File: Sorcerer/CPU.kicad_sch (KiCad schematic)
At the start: 35 parts

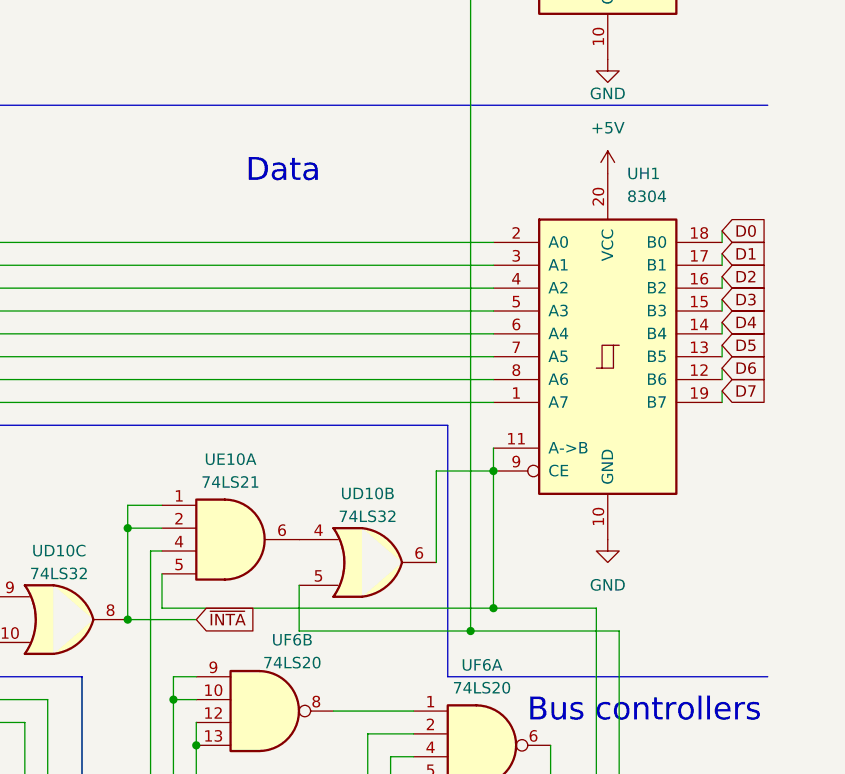
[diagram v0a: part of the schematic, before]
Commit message: Fix some issues I found.
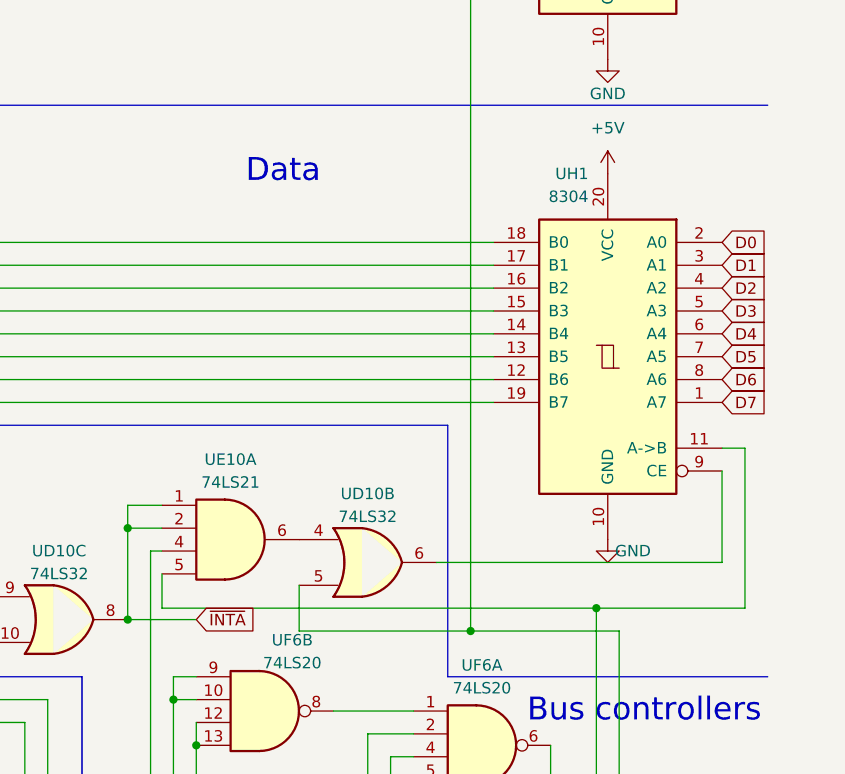
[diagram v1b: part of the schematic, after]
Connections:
- net D0: now also UH1.2 (A0); no longer UH1.18 (B0)
- net D1: now also UH1.3 (A1); no longer UH1.17 (B1)
- net D2: now also UH1.4 (A2); no longer UH1.16 (B2)
- net D3: now also UH1.5 (A3); no longer UH1.15 (B3)
- net D4: now also UH1.6 (A4); no longer UH1.14 (B4)
- net D5: now also UH1.7 (A5); no longer UH1.13 (B5)
- net D6: now also UH1.8 (A6); no longer UH1.12 (B6)
- net D7: now also UH1.1 (A7); no longer UH1.19 (B7)
- net ~{DBUS_OUT}: no longer UD10.6, UH1.9 (CE)
- net at UE2.10 (D_{6}): now also UH1.12 (B6); no longer UH1.8 (A6)
- net at UE2.12 (D_{2}): now also UH1.16 (B2); no longer UH1.4 (A2)
- net at UE2.13 (D_{7}): now also UH1.19 (B7); no longer UH1.1 (A7)
- net at UE2.14 (D_{0}): now also UH1.18 (B0); no longer UH1.2 (A0)
- net at UE2.15 (D_{1}): now also UH1.17 (B1); no longer UH1.3 (A1)
- net at UE2.7 (D_{4}): now also UH1.14 (B4); no longer UH1.6 (A4)
- net at UE2.8 (D_{3}): now also UH1.15 (B3); no longer UH1.5 (A3)
- net at UE2.9 (D_{5}): now also UH1.13 (B5); no longer UH1.7 (A5)
- new net: UD10.6, UH1.9 (CE)
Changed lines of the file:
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@@
 	)
 	(junction
-		(at 375.92 157.48)
-		(diameter 0)
-		(color 0 0 0 0)
-	)
-	(junction
 		(at 298.45 232.41)
 		(diameter 0)
@@
 	)
 	(junction
+		(at 387.35 172.72)
+		(diameter 0)
+		(color 0 0 0 0)
+	)
+	(junction
 		(at 260.35 257.81)
 		(diameter 0)
@@
 	)
 	(junction
-		(at 375.92 172.72)
-		(diameter 0)
-		(color 0 0 0 0)
-	)
-	(junction
 		(at 234.95 175.26)
 		(diameter 0)
@@
 	(wire
 		(pts
+			(xy 401.32 154.94) (xy 403.86 154.94)
+		)
+		(stroke
+			(width 0)
+			(type default)
+		)
+	)
+	(wire
+		(pts
 			(xy 264.16 255.27) (xy 267.97 255.27)
 		)
@@
 	(wire
 		(pts
-			(xy 387.35 172.72) (xy 375.92 172.72)
+			(xy 339.09 172.72) (xy 387.35 172.72)
 		)
 		(stroke
@@
 	(wire
 		(pts
-			(xy 401.32 139.7) (xy 401.32 138.43)
-		)
-		(stroke
-			(width 0)
-			(type default)
-		)
-	)
-	(wire
-		(pts
 			(xy 275.59 144.78) (xy 262.89 144.78)
 		)
@@
 	(wire
 		(pts
-			(xy 369.57 157.48) (xy 375.92 157.48)
-		)
-		(stroke
-			(width 0)
-			(type default)
-		)
-	)
-	(wire
-		(pts
 			(xy 156.21 252.73) (xy 156.21 245.11)
 		)
@@
 	(wire
 		(pts
+			(xy 369.57 167.64) (xy 401.32 167.64)
+		)
+		(stroke
+			(width 0)
+			(type default)
+		)
+	)
+	(wire
+		(pts
 			(xy 367.03 191.77) (xy 367.03 207.01)
 		)
@@
 	(wire
 		(pts
-			(xy 401.32 142.24) (xy 401.32 140.97)
-		)
-		(stroke
-			(width 0)
-			(type default)
-		)
-	)
-	(wire
-		(pts
 			(xy 267.97 152.4) (xy 262.89 152.4)
 		)
@@
 	(wire
 		(pts
-			(xy 401.32 149.86) (xy 401.32 148.59)
-		)
-		(stroke
-			(width 0)
-			(type default)
-		)
-	)
-	(wire
-		(pts
 			(xy 222.25 137.16) (xy 237.49 137.16)
 		)
@@
 	(wire
 		(pts
-			(xy 375.92 172.72) (xy 375.92 157.48)
-		)
-		(stroke
-			(width 0)
-			(type default)
-		)
-	)
-	(wire
-		(pts
 			(xy 265.43 27.94) (xy 265.43 154.94)
 		)
@@
 	(wire
 		(pts
-			(xy 401.32 137.16) (xy 401.32 135.89)
-		)
-		(stroke
-			(width 0)
-			(type default)
-		)
-	)
-	(wire
-		(pts
 			(xy 99.06 26.67) (xy 99.06 24.13)
 		)
@@
 	(wire
 		(pts
-			(xy 401.32 134.62) (xy 401.32 133.35)
-		)
-		(stroke
-			(width 0)
-			(type default)
-		)
-	)
-	(wire
-		(pts
 			(xy 219.71 142.24) (xy 237.49 142.24)
 		)
@@
 	(wire
 		(pts
-			(xy 401.32 132.08) (xy 401.32 130.81)
-		)
-		(stroke
-			(width 0)
-			(type default)
-		)
-	)
-	(wire
-		(pts
 			(xy 336.55 222.25) (xy 336.55 250.19)
 		)
@@
 	(wire
 		(pts
-			(xy 369.57 167.64) (xy 369.57 157.48)
-		)
-		(stroke
-			(width 0)
-			(type default)
-		)
-	)
-	(wire
-		(pts
 			(xy 280.67 35.56) (xy 280.67 139.7)
 		)
@@
 	(wire
 		(pts
+			(xy 403.86 154.94) (xy 403.86 172.72)
+		)
+		(stroke
+			(width 0)
+			(type default)
+		)
+	)
+	(wire
+		(pts
 			(xy 25.4 45.72) (xy 35.56 45.72)
 		)
@@
 	(wire
 		(pts
-			(xy 401.32 147.32) (xy 401.32 146.05)
-		)
-		(stroke
-			(width 0)
-			(type default)
-		)
-	)
-	(wire
-		(pts
 			(xy 303.53 232.41) (xy 303.53 241.3)
 		)
@@
 	(wire
 		(pts
+			(xy 401.32 167.64) (xy 401.32 157.48)
+		)
+		(stroke
+			(width 0)
+			(type default)
+		)
+	)
+	(wire
+		(pts
 			(xy 323.85 207.01) (xy 367.03 207.01)
 		)
@@
 	(wire
 		(pts
-			(xy 401.32 144.78) (xy 401.32 143.51)
+			(xy 403.86 172.72) (xy 387.35 172.72)
 		)
 		(stroke
@@
 	(wire
 		(pts
-			(xy 375.92 157.48) (xy 375.92 154.94)
-		)
-		(stroke
-			(width 0)
-			(type default)
-		)
-	)
-	(wire
-		(pts
 			(xy 127 57.15) (xy 127 58.42)
 		)
@@
 	(wire
 		(pts
-			(xy 339.09 172.72) (xy 375.92 172.72)
-		)
-		(stroke
-			(width 0)
-			(type default)
-		)
-	)
-	(wire
-		(pts
 			(xy 354.33 175.26) (xy 373.38 175.26)
 		)
@@
 	(global_label "D7"
 		(shape input)
-		(at 401.32 148.59 0)
+		(at 401.32 149.86 0)
 		(fields_autoplaced yes)
 		(effects
@@
 		)
 		(property "Intersheetrefs" "${INTERSHEET_REFS}"
-			(at 406.7847 148.59 0)
+			(at 406.7847 149.86 0)
 			(effects
 				(font
@@
 	(global_label "D1"
 		(shape input)
-		(at 401.32 133.35 0)
+		(at 401.32 134.62 0)
 		(fields_autoplaced yes)
 		(effects
@@
 		)
 		(property "Intersheetrefs" "${INTERSHEET_REFS}"
-			(at 406.7847 133.35 0)
+			(at 406.7847 134.62 0)
 			(effects
 				(font
@@
 	(global_label "D2"
 		(shape input)
-		(at 401.32 135.89 0)
+		(at 401.32 137.16 0)
 		(fields_autoplaced yes)
 		(effects
@@
 		)
 		(property "Intersheetrefs" "${INTERSHEET_REFS}"
-			(at 406.7847 135.89 0)
+			(at 406.7847 137.16 0)
 			(effects
 				(font
@@
 	(global_label "D0"
 		(shape input)
-		(at 401.32 130.81 0)
+		(at 401.32 132.08 0)
 		(fields_autoplaced yes)
 		(effects
@@
 		)
 		(property "Intersheetrefs" "${INTERSHEET_REFS}"
-			(at 406.7847 130.81 0)
+			(at 406.7847 132.08 0)
 			(effects
 				(font
@@
 	(global_label "D6"
 		(shape input)
-		(at 401.32 146.05 0)
+		(at 401.32 147.32 0)
 		(fields_autoplaced yes)
 		(effects
@@
 		)
 		(property "Intersheetrefs" "${INTERSHEET_REFS}"
-			(at 406.7847 146.05 0)
+			(at 406.7847 147.32 0)
 			(effects
 				(font
@@
 	(global_label "D5"
 		(shape input)
-		(at 401.32 143.51 0)
+		(at 401.32 144.78 0)
 		(fields_autoplaced yes)
 		(effects
@@
 		)
 		(property "Intersheetrefs" "${INTERSHEET_REFS}"
-			(at 406.7847 143.51 0)
+			(at 406.7847 144.78 0)
 			(effects
 				(font
@@
 	(global_label "D3"
 		(shape input)
-		(at 401.32 138.43 0)
+		(at 401.32 139.7 0)
 		(fields_autoplaced yes)
 		(effects
@@
 		)
 		(property "Intersheetrefs" "${INTERSHEET_REFS}"
-			(at 406.7847 138.43 0)
+			(at 406.7847 139.7 0)
 			(effects
 				(font
@@
 	(global_label "D4"
 		(shape input)
-		(at 401.32 140.97 0)
+		(at 401.32 142.24 0)
 		(fields_autoplaced yes)
 		(effects
@@
 		)
 		(property "Intersheetrefs" "${INTERSHEET_REFS}"
-			(at 406.7847 140.97 0)
+			(at 406.7847 142.24 0)
 			(effects
 				(font
@@
 		(on_board yes)
 		(dnp no)
-		(fields_autoplaced yes)
 		(property "Reference" "#PWR0107"
 			(at 388.62 171.45 0)
@@
 		)
 		(property "Value" "GND"
-			(at 388.62 170.18 0)
+			(at 391.414 166.37 0)
 			(effects
 				(font
@@
 		(lib_id "TholinsStuff:8304")
 		(at 388.62 144.78 0)
+		(mirror y)
 		(unit 1)
 		(exclude_from_sim no)
@@
 		(on_board yes)
 		(dnp no)
-		(fields_autoplaced yes)
 		(property "Reference" "UH1"
-			(at 390.7633 124.46 0)
+			(at 386.4767 124.46 0)
 			(effects
 				(font
@@
 		)
 		(property "Value" "8304"
-			(at 390.7633 127 0)
+			(at 386.4767 127 0)
 			(effects
 				(font
